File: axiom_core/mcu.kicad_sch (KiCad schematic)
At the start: 30 parts, among them SW2 BOOT, SW3 RST, U5 PCA9536D, U6 ESP32-S3, U7 W25Q128JVSIQ, Y1 TROQ RG40000421, Y2 EPSON Q13FC13500004

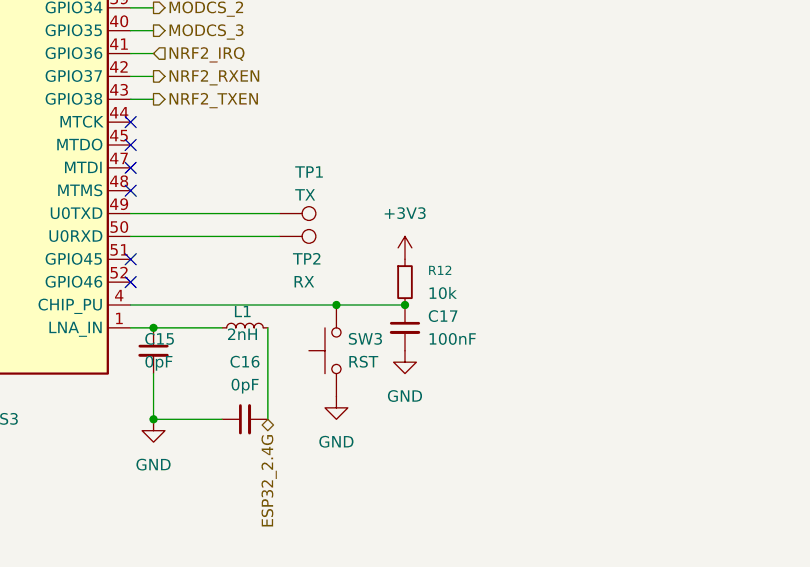
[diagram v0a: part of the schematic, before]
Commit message: upload
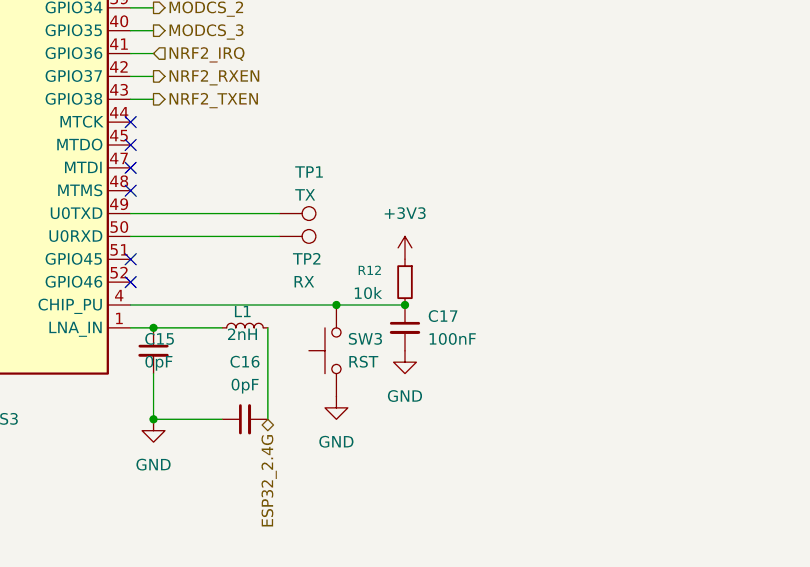
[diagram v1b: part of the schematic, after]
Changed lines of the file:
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@@
 		(lib_id "Device:R_Small")
 		(at 158.75 147.32 0)
+		(mirror y)
 		(unit 1)
 		(exclude_from_sim no)
@@
 		(on_board yes)
 		(dnp no)
-		(fields_autoplaced yes)
 		(property "Reference" "R12"
-			(at 161.29 146.0499 0)
+			(at 156.21 146.0499 0)
 			(effects
 				(font
@@
 		)
 		(property "Value" "10k"
-			(at 161.29 148.5899 0)
+			(at 156.21 148.5899 0)
 			(effects
 				(font
